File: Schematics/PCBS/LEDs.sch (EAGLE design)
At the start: 16 parts, among them IC1 ATMEGA328P-AU, Q1 TRANSISTOR-FET_DMN2004K, Q2 TRANSISTOR-FET_DMN2004K, Q3 TRANSISTOR-FET_DMN2004K, Q4 TRANSISTOR-FET_DMN2004K, Q5 TRANSISTOR-FET_DMN2004K, Q6 TRANSISTOR-FET_DMN2004K, Q7 TRANSISTOR-FET_DMN2004K, Q8 TRANSISTOR-FET_DMN2004K, Q9 TRANSISTOR-FET_DMN2004K, U1 LT1763CS8-3.3#TRPBF

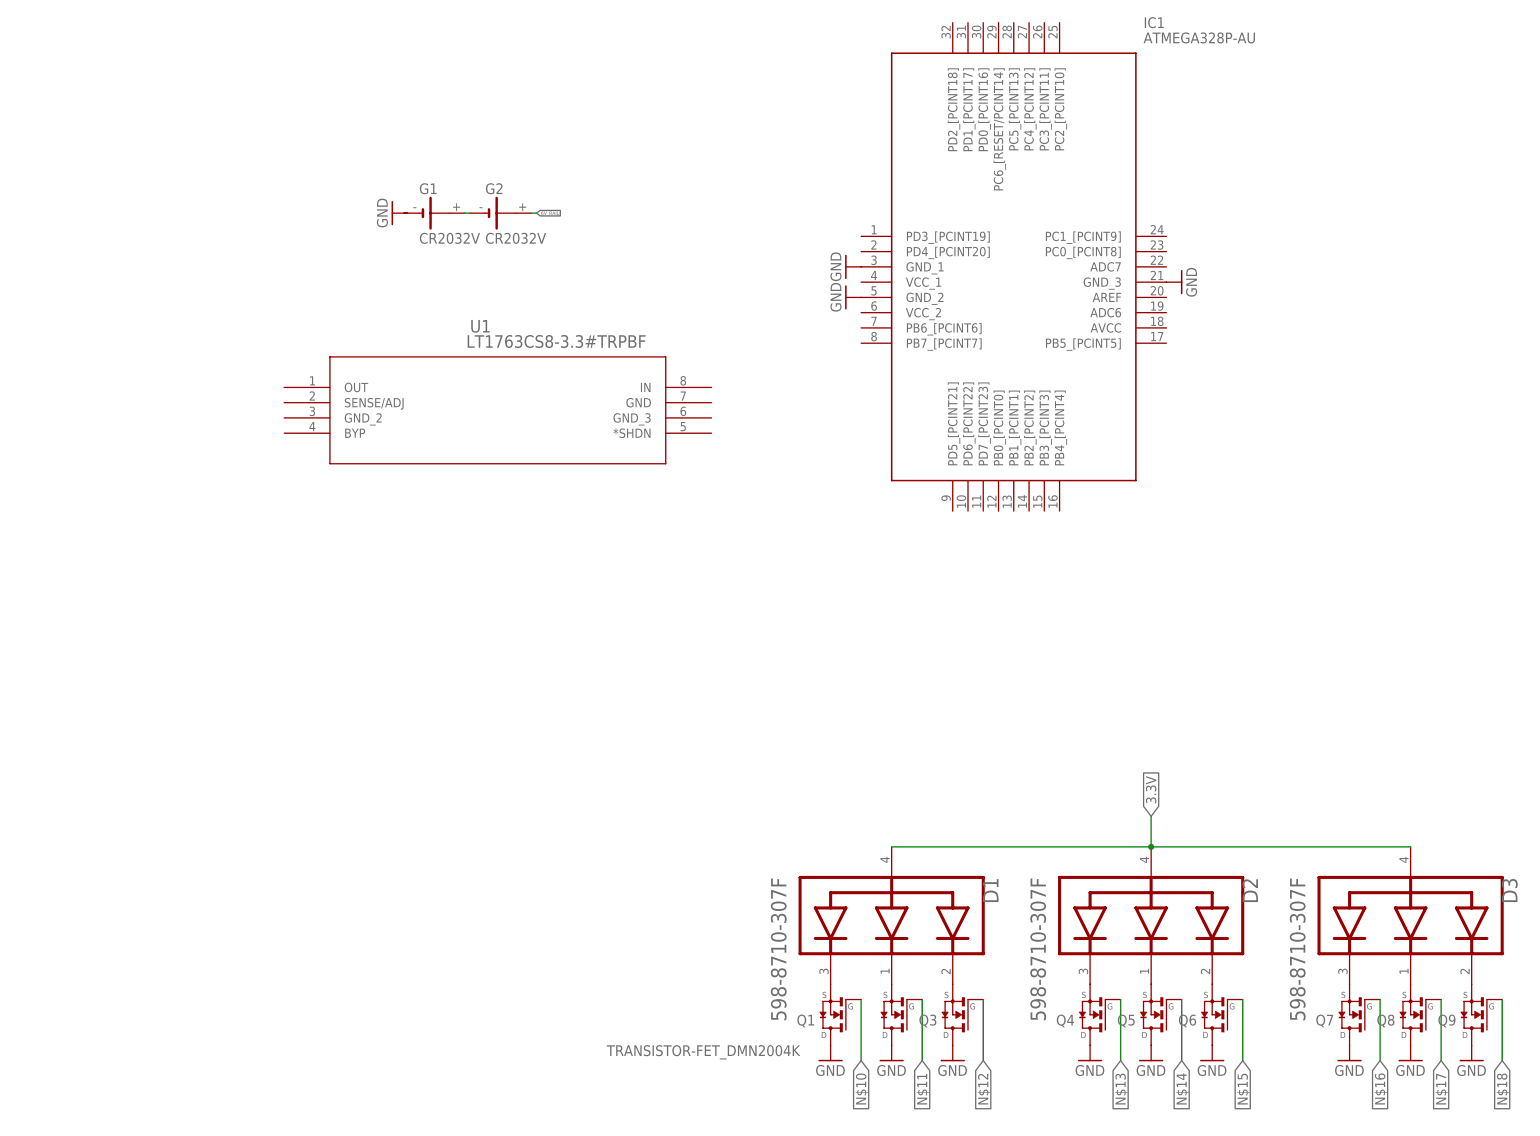
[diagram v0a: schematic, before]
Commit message: update power Rail
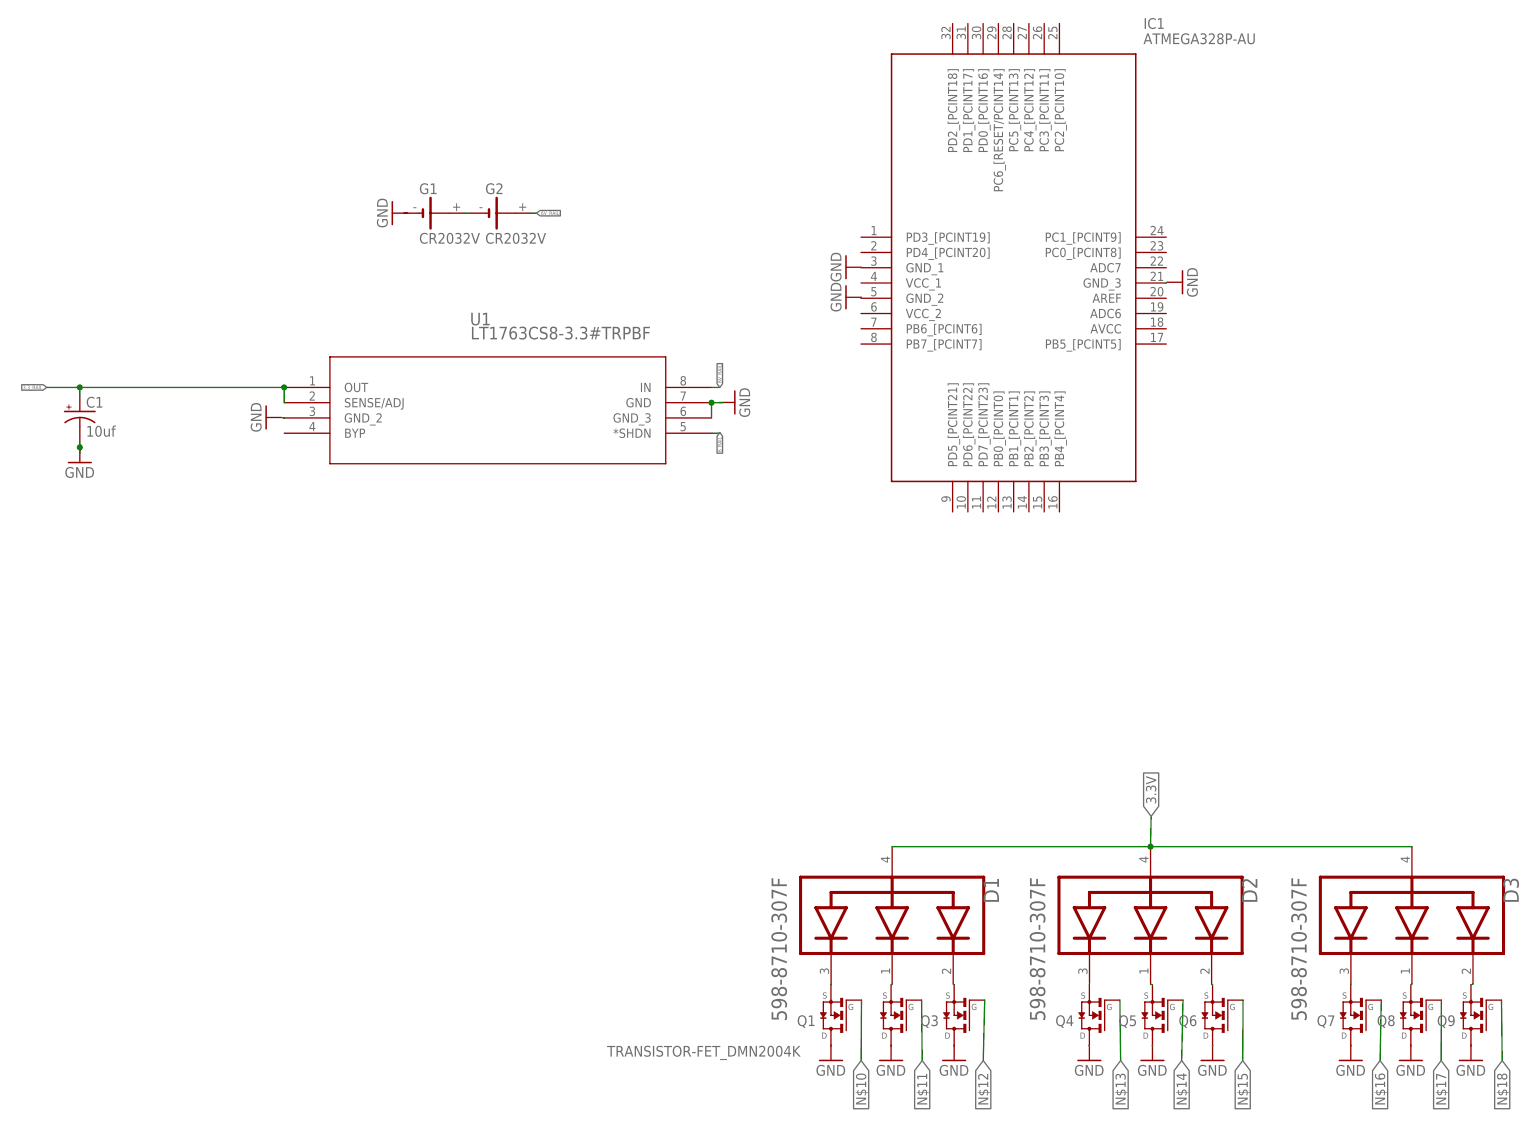
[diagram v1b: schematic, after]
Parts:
- added C1: 10uf, adafruit:CPOL-USE1.8-4
- D1, D2, D3: SPICEPREFIX (none) -> E
- G1, G2: SPICEPREFIX (none) -> J
- IC1, U1: SPICEPREFIX (none) -> X
- Q1, Q2, Q3, Q4, Q5, Q6, Q7, Q8, Q9: SPICEPREFIX (none) -> Q
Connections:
- new net 3.3_RAIL: C1.+, U1.OUT, U1.SENSE/ADJ
- new net 6_RAIL: U1.*SHDN
- new net N$20: U1.GND, U1.GND_3
- net 6V_RAIL: now also U1.IN
- net GND: now also C1.-, U1.GND_2
